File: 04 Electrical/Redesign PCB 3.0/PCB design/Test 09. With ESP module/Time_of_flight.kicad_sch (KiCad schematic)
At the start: 4 parts, among them U10 LP5907MFX-2.8/NOPB, U11 VL53L0CXV0DH/1

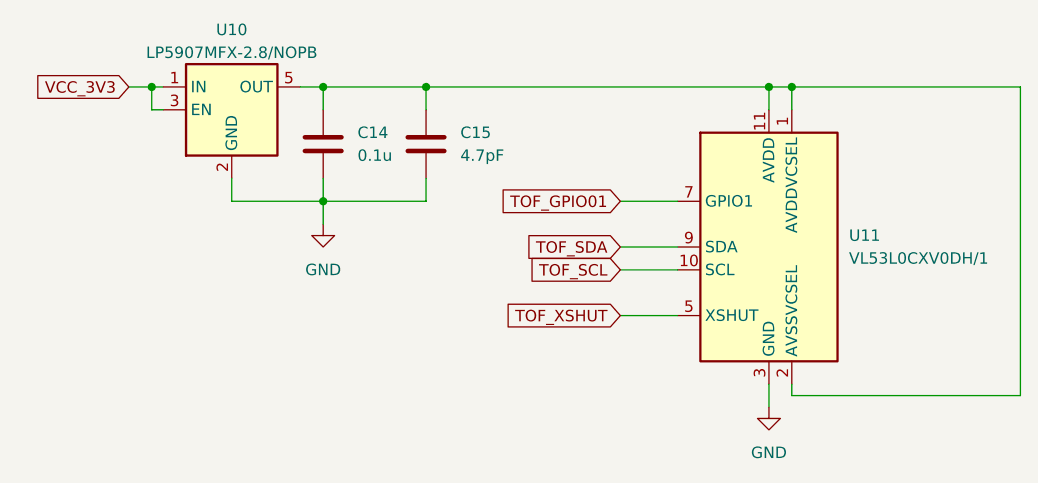
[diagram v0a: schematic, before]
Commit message: Routing PCB test 9
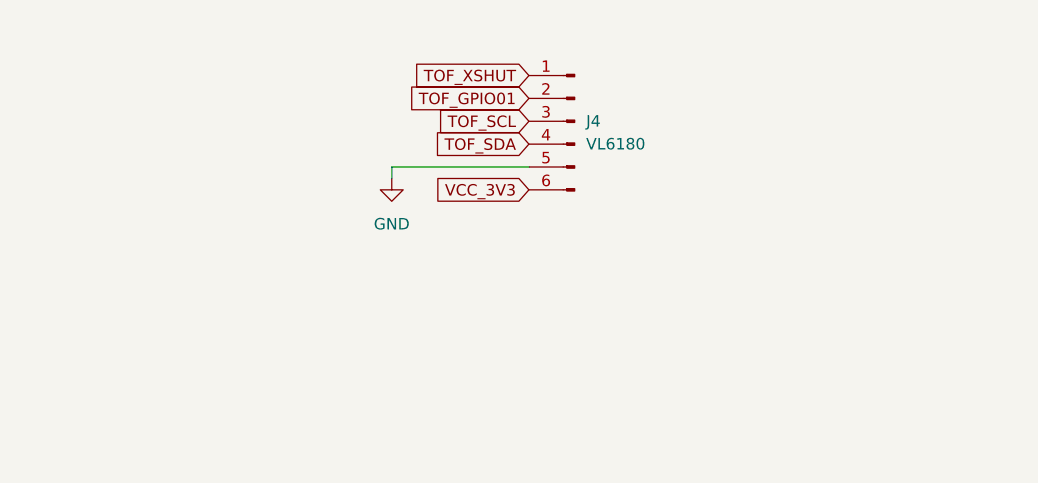
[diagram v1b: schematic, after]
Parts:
- removed C14: 0.1u, Capacitor_SMD:C_0603_1608Metric, symbol Device:C
- removed C15: 4.7pF, Capacitor_SMD:C_0603_1608Metric, symbol Device:C
- removed U10: LP5907MFX-2.8/NOPB, Package_TO_SOT_SMD:SOT-23-5, symbol Regulator_Linear:LP5907MFX-2.8
- removed U11: VL53L0CXV0DH/1, Sensor_Distance:ST_VL53L1x, symbol Sensor_Distance:VL53L0CXV0DH1
- added J4: VL6180, Connector_PinHeader_2.00mm:PinHeader_1x06_P2.00mm_Vertical, symbol Connector:Conn_01x06_Pin
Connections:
- net GND: now also J4.5 (Pin_5)
- net TOF_GPIO01: now also J4.2 (Pin_2)
- net TOF_SCL: now also J4.3 (Pin_3)
- net TOF_SDA: now also J4.4 (Pin_4)
- net TOF_XSHUT: now also J4.1 (Pin_1)
- net VCC_3V3: now also J4.6 (Pin_6)
